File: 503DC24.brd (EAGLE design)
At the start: 2 parts

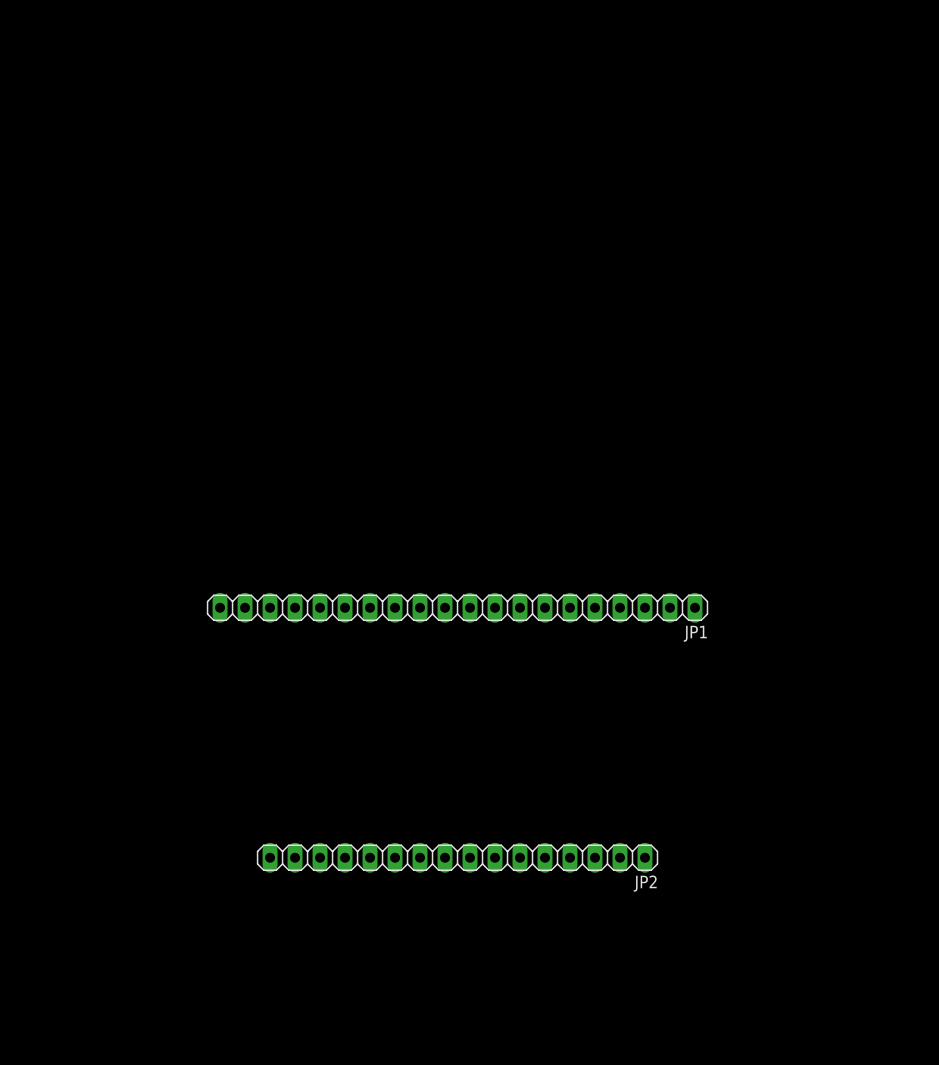
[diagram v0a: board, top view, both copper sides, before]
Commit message: Adding Board Schematic, Layout, & additional files for design
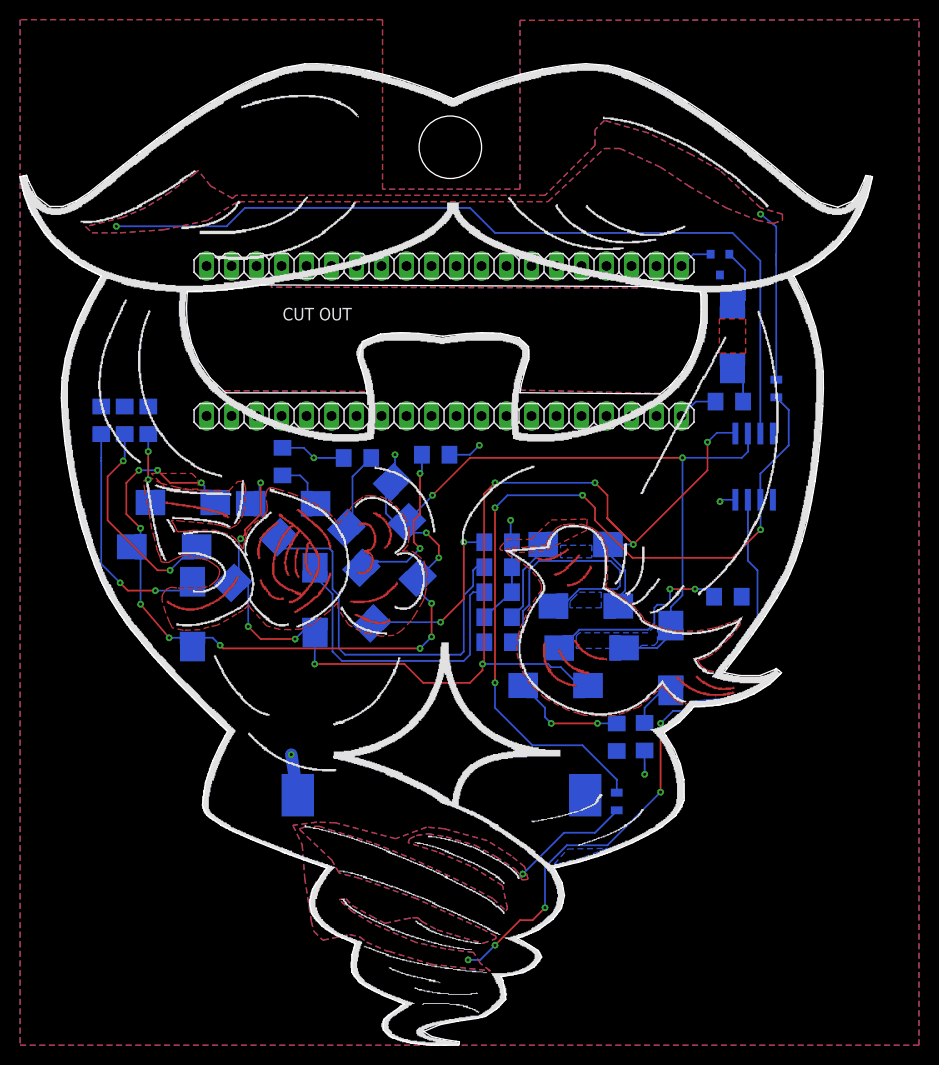
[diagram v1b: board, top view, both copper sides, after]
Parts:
- removed JP1: (no value), pinhead:1X20
- removed JP2: (no value), pinhead:1X16
- added BAT1: BU2032BU2032SM, Electromechanical:BU2032SM
- added D1, D10, D11, D12, D13, D14, D15, D16, D2, D3, D4, D5, D6, D7, D8: (no value), LED:LED-REV-MNT-SMALLSILK
- added JP3: Top header, pinhead:1X20
- added JP4: Bottom header, pinhead:1X20
- added Q1: 200mA/50V, SparkFun-DiscreteSemi:SOT23-3
- added R1, R10, R11, R12, R13, R14, R15, R16, R2, R3, R4, R5, R6, R7, R8: (no value), SparkFun-Passives:1206
- added R17, R18: 10M, SparkFun-Passives:0805
- added U1: Tiny85-20-SMT, SparkFun-DigitalIC:SO08-EIAJ
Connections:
- removed net A00: JP2.9
- removed net A01: JP2.8
- removed net A02: JP2.7
- removed net A03: JP2.6
- removed net A04: JP2.5
- removed net A05: JP2.4
- removed net A06: JP2.3
- removed net A07: JP2.2
- removed net A08: JP2.1
- removed net GPIO09: JP1.15
- removed net GPIO10: JP1.6
- removed net GPIO11: JP1.7
- removed net GPIO12: JP1.8
- removed net GPIO13: JP1.9
- removed net GPIO14: JP1.10
- removed net GPIO15: JP1.11
- removed net GPIO16: JP1.12
- removed net GPIO17: JP1.13
- removed net GPIO18: JP1.14
- removed net GPIO24: JP2.10
- new net CAP0: R17.1, U1.3
- new net CAP1: R18.1, U1.7
- new net GND1: BAT1.P-, R11.2, R12.2, R15.2, R16.2, R3.2, R4.2, R7.2, R8.2, U1.4
- new net N$14: D10.A, R10.2
- new net N$15: D12.C, R12.1
- new net N$16: D11.C, R11.1
- new net N$17: D8.C, R8.1
- new net N$18: D7.C, R7.1
- new net N$2: D2.A, R2.2
- new net N$21: D13.A, R13.2
- new net N$22: D14.A, R14.2
- new net N$27: D1.A, Q1.2
- new net N$3: D3.C, R3.1
- new net N$30: D1.C, R1.2
- new net N$4: D4.C, R4.1
- new net N$5: D5.A, R5.2
- new net N$6: D6.A, R6.2
- new net N$7: D16.C, R16.1
- new net N$8: D15.C, R15.1
- new net PWM0: D11.A, D13.C, D15.A, D3.A, D5.C, D7.A, U1.5
- new net PWM1: D10.C, D12.A, D14.C, D16.A, D2.C, D4.A, D6.C, D8.A, U1.6
- new net SENSE: R17.2, R18.2, U1.2
- new net VCC1: BAT1.P+, Q1.3, R10.1, R13.1, R14.1, R2.1, R5.1, R6.1, U1.8
- net GND: now also JP4.1, R1.1; no longer JP1.4
- net VCC: now also JP3.1, Q1.1; no longer JP1.3
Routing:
- net PWM1: track 0.00 -> 145.9 mm, vias 0 -> 15
- net PWM0: track 0.00 -> 129.8 mm, vias 0 -> 10
- net CAP1: track 0.00 -> 103.6 mm, vias 0 -> 2
- net CAP0: track 0.00 -> 85.8 mm, vias 0 -> 6
- net SENSE: track 0.00 -> 84.3 mm, vias 0 -> 4
- net N$18: track 0.00 -> 39.6 mm
- net N$16: track 0.00 -> 30.6 mm
- net GND1: track 0.00 -> 29.5 mm, vias 0 -> 6
- net N$5: track 0.00 -> 26.3 mm
- net N$22: track 0.00 -> 24.1 mm, vias 0 -> 2
- net N$6: track 0.00 -> 21.3 mm, vias 0 -> 2
- net N$14: track 0.00 -> 19.7 mm, vias 0 -> 2
- net N$15: track 0.00 -> 18.0 mm, vias 0 -> 2
- net N$17: track 0.00 -> 17.0 mm, vias 0 -> 2
- net N$21: track 0.00 -> 11.3 mm, vias 0 -> 2
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- added copper zone on layer 1, net CAP0
- added copper zone on layer 16, net CAP0
- added copper zone on layer 1, net CAP1
- added copper zone on layer 16, net CAP1
- added copper zone on layer 1, net GND1
- added copper zone on layer 1, net N$1
- added copper zone on layer 16, net N$10
- added copper zone on layer 16, net N$11
- added copper zone on layer 16, net N$12
- added copper zone on layer 1, net N$13
- added copper zone on layer 16, net N$19
- added copper zone on layer 1, net N$20
- added copper zone on layer 1, net N$23
- added copper zone on layer 16, net N$23
- added copper zone on layer 1, net N$24
- added copper zone on layer 16, net N$24
- added copper zone on layer 1, net N$25
- added copper zone on layer 16, net N$25
- added copper zone on layer 1, net N$26
- added copper zone on layer 1, net N$28
- added copper zone on layer 1, net N$9
- added copper zone on layer 16, net VCC1
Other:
- board outline added: 86.6 x 99.8 mm
- board text added: "Artwork by @remeranAuthor"
- board text added: "CUT OUT"
- board text added: "DC 503"
- board text added: "Made In PDX"
- board text added: "Up to the minute details at http://503.party"
- board text added: "Warthog9 put a bird on it"
- board text added: "cordially invites you to put your bird on our little schindig"
